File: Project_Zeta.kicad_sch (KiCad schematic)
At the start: 14 parts, among them J1 Conn_01x20, J2 Conn_01x20, J3 Screw_Terminal_01x02, J4 Screw_Terminal_01x04, J5 Screw_Terminal_01x04, J6 Screw_Terminal_01x04, J7 Screw_Terminal_01x04, J8 Conn_01x03, J9 Conn_01x03

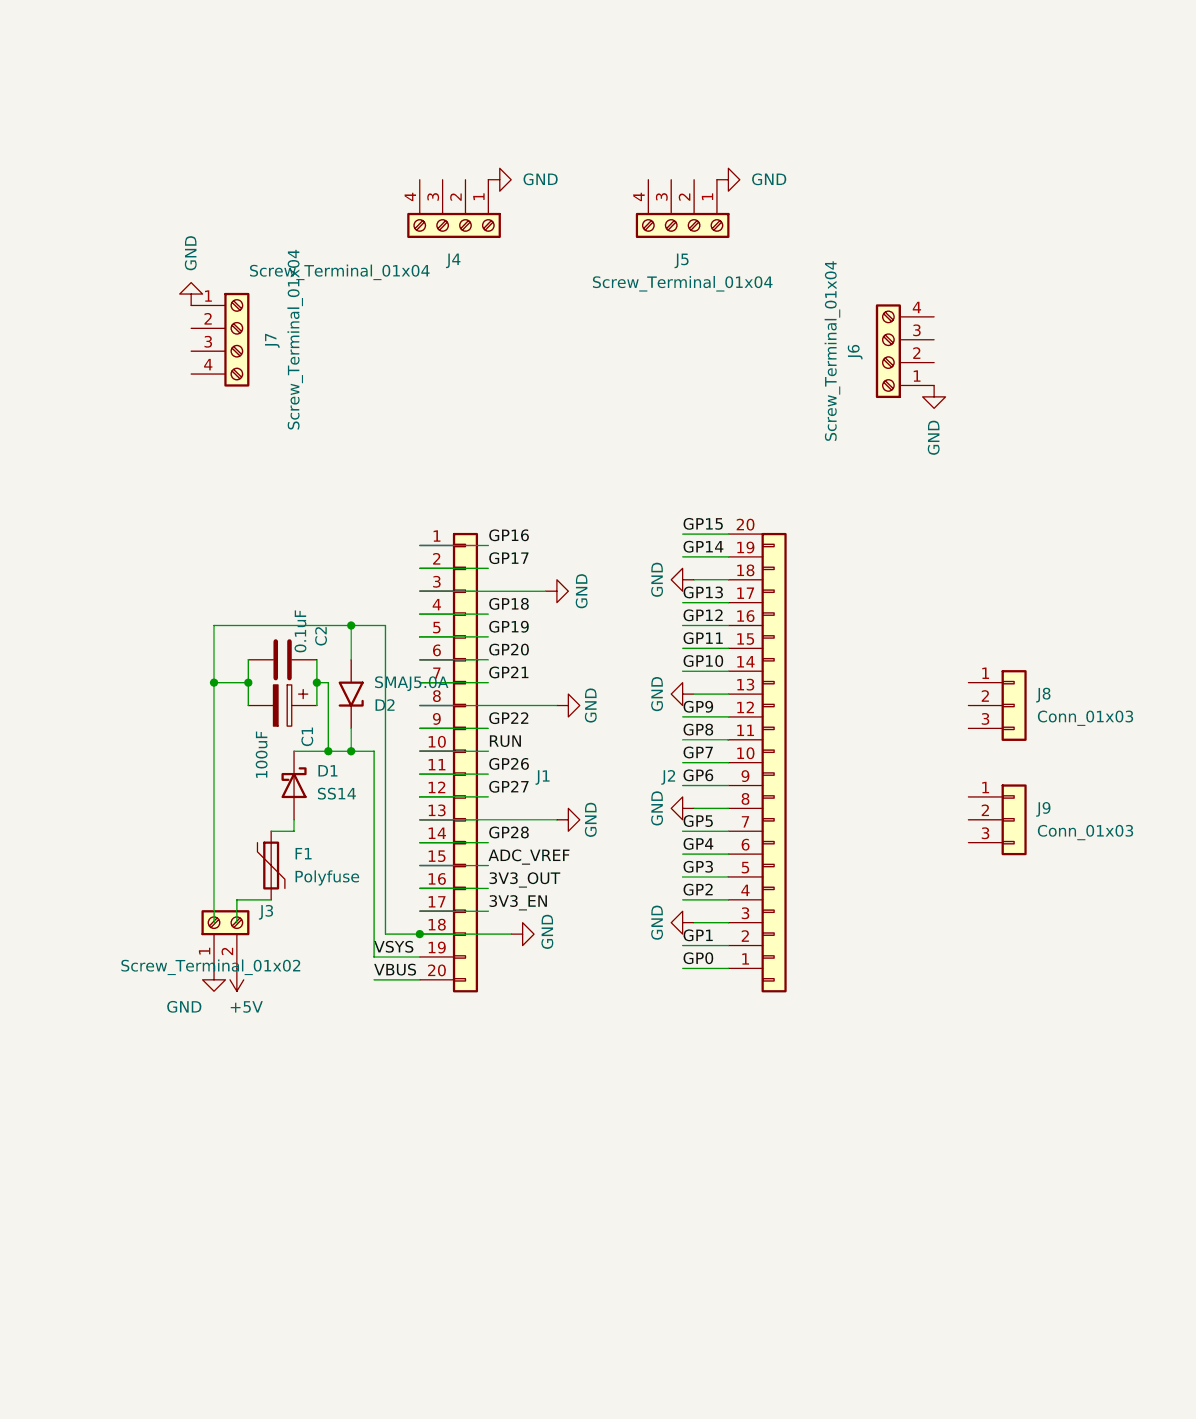
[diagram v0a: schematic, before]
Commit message: Init with Rev 1.1
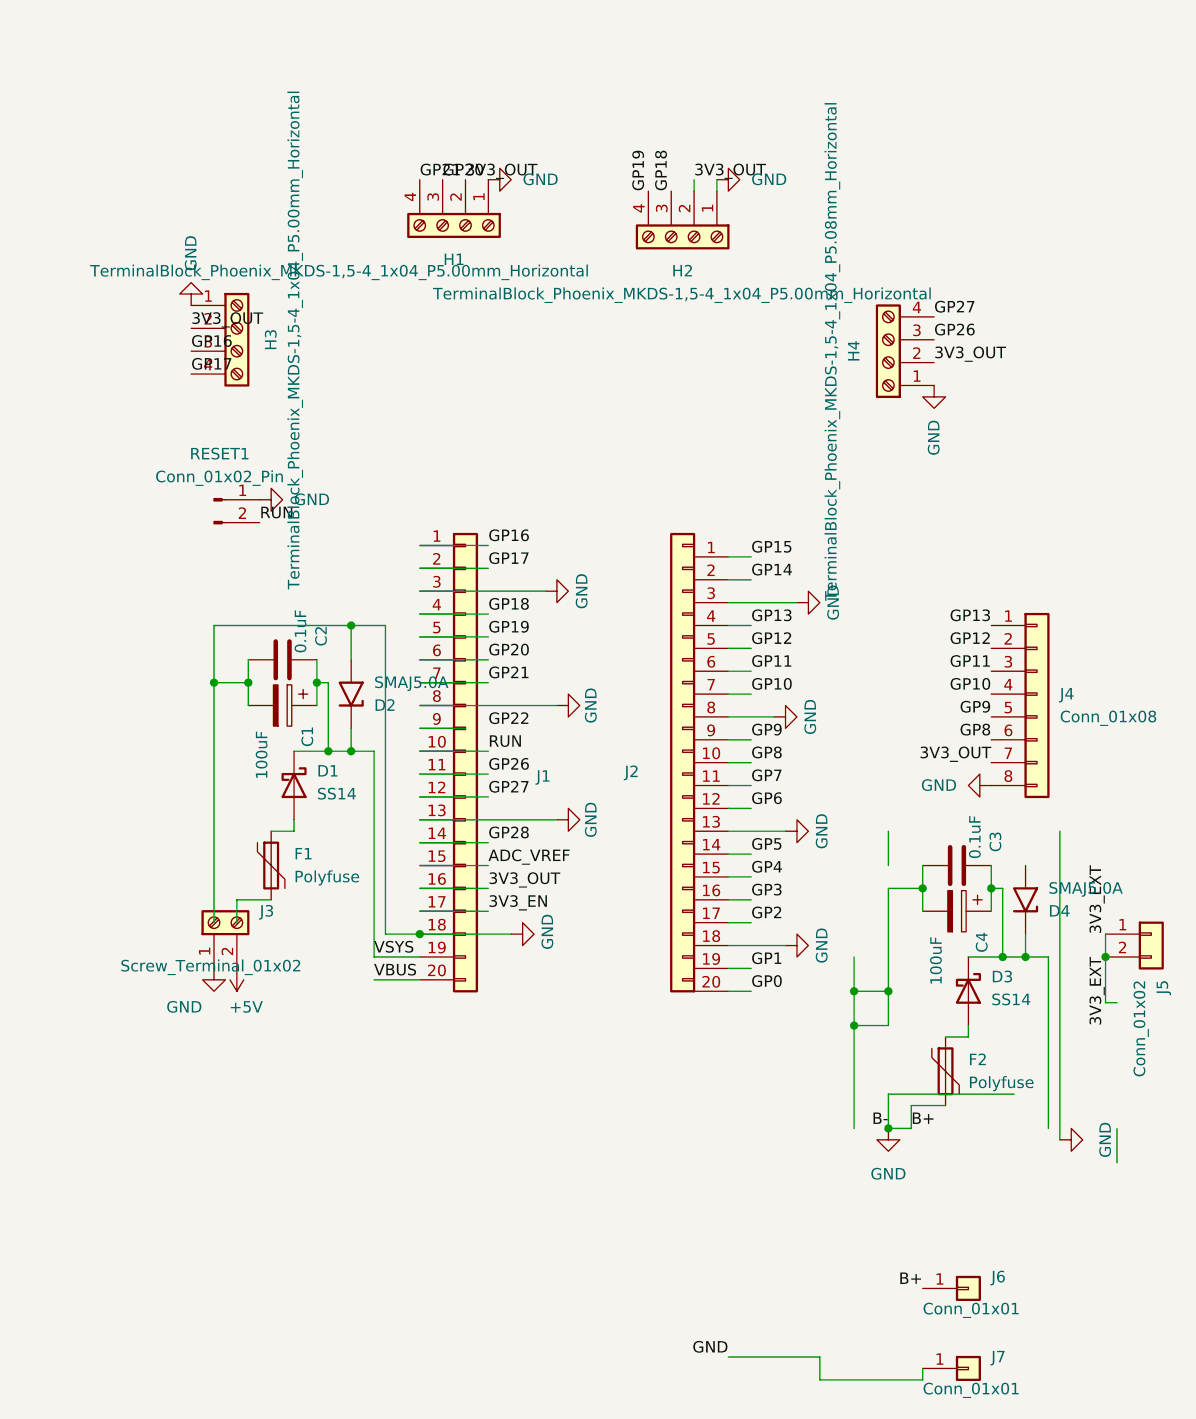
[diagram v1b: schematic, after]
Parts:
- removed J8, J9: Conn_01x03, Connector_PinHeader_2.54mm:PinHeader_1x03_P2.54mm_Vertical, symbol Connector_Generic:Conn_01x03
- added C3: 0.1uF, symbol Device:C
- added C4: 100uF, symbol Device:C_Polarized
- added D3: SS14, Diode_SMD:D_SMA, symbol Diode:SS14
- added D4: SMAJ5.0A, Diode_SMD:D_SMA, symbol Diode:SMAJ5.0A
- added F2: Polyfuse, symbol Device:Polyfuse
- added J4: Conn_01x08, Connector_PinHeader_2.54mm:PinHeader_1x08_P2.54mm_Horizontal, symbol Connector_Generic:Conn_01x08
- added J5: Conn_01x02, Connector_PinHeader_2.54mm:PinHeader_1x02_P2.54mm_Horizontal, symbol Connector_Generic:Conn_01x02
- added J6, J7: Conn_01x01, Connector_Wire:SolderWire-0.25sqmm_1x01_D0.65mm_OD2mm, symbol Connector_Generic:Conn_01x01
- added RESET1: Conn_01x02_Pin, Connector_PinHeader_2.54mm:PinHeader_1x02_P2.54mm_Vertical, symbol Connector:Conn_01x02_Pin
- H1: renamed from J4; value Screw_Terminal_01x04 -> TerminalBlock_Phoenix_MKDS-1,5-4_1x04_P5.00mm_Horizontal; footprint (none) -> TerminalBlock_Phoenix_MKDS-1,5-4_1x04_P5.00mm_Horizontal
- H2: renamed from J5; value Screw_Terminal_01x04 -> TerminalBlock_Phoenix_MKDS-1,5-4_1x04_P5.00mm_Horizontal; footprint (none) -> TerminalBlock_Phoenix_MKDS-1,5-4_1x04_P5.00mm_Horizontal
- H3: renamed from J7; value Screw_Terminal_01x04 -> TerminalBlock_Phoenix_MKDS-1,5-4_1x04_P5.00mm_Horizontal; footprint (none) -> TerminalBlock_Phoenix_MKDS-1,5-4_1x04_P5.00mm_Horizontal
- H4: renamed from J6; value Screw_Terminal_01x04 -> TerminalBlock_Phoenix_MKDS-1,5-4_1x04_P5.08mm_Horizontal; footprint (none) -> TerminalBlock_Phoenix_MKDS-1,5-4_1x04_P5.00mm_Horizontal
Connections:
- net 3V3_OUT: now also H1.2 (Pin_2), H2.2 (Pin_2), H3.2 (Pin_2), H4.2 (Pin_2), J4.7 (Pin_7)
- net GND: now also F2.2, J4.8 (Pin_8), J6.1 (Pin_1), J7.1 (Pin_1), RESET1.1 (Pin_1)
- net GP0: now also J2.20 (Pin_20); no longer J2.1 (Pin_1)
- net GP1: now also J2.19 (Pin_19); no longer J2.2 (Pin_2)
- net GP10: now also J2.7 (Pin_7), J4.4 (Pin_4); no longer J2.14 (Pin_14)
- net GP11: now also J2.6 (Pin_6), J4.3 (Pin_3); no longer J2.15 (Pin_15)
- net GP12: now also J2.5 (Pin_5), J4.2 (Pin_2); no longer J2.16 (Pin_16)
- net GP13: now also J2.4 (Pin_4), J4.1 (Pin_1); no longer J2.17 (Pin_17)
- net GP14: now also J2.2 (Pin_2); no longer J2.19 (Pin_19)
- net GP15: now also J2.1 (Pin_1); no longer J2.20 (Pin_20)
- net GP16: now also H3.3 (Pin_3)
- net GP17: now also H3.4 (Pin_4)
- net GP18: now also H2.3 (Pin_3)
- net GP19: now also H2.4 (Pin_4)
- net GP2: now also J2.17 (Pin_17); no longer J2.4 (Pin_4)
- net GP20: now also H1.3 (Pin_3)
- net GP21: now also H1.4 (Pin_4)
- net GP22: no longer J1.9 (GP22)
- net GP26: now also H4.3 (Pin_3)
- net GP27: now also H4.4 (Pin_4)
- net GP3: now also J2.16 (Pin_16); no longer J2.5 (Pin_5)
- net GP4: now also J2.15 (Pin_15); no longer J2.6 (Pin_6)
- net GP5: now also J2.14 (Pin_14); no longer J2.7 (Pin_7)
- net GP6: now also J2.12 (Pin_12); no longer J2.9 (Pin_9)
- net GP7: now also J2.11 (Pin_11); no longer J2.10 (Pin_10)
- net GP8: now also J2.10 (Pin_10), J4.6 (Pin_6); no longer J2.11 (Pin_11)
- net GP9: now also J2.9 (Pin_9), J4.5 (Pin_5); no longer J2.12 (Pin_12)
- net RUN: now also RESET1.2 (Pin_2)
- new net: C3.1, C4.1, D3.1 (K), D4.1 (A1)
- new net: C3.2, C4.2
- new net: D3.2 (A), F2.1
- new net 3V3_EXT: J5.1 (Pin_1), J5.2 (Pin_2)
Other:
- title: (none) -> Project Zeta
- moved on the sheet: H2, J2
